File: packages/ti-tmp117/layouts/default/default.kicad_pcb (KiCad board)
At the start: 2 copper layers, 4 parts

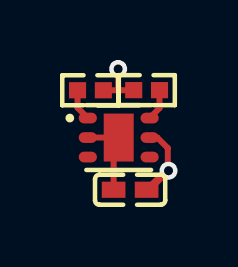
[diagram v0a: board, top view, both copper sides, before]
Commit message: rebuild all packages
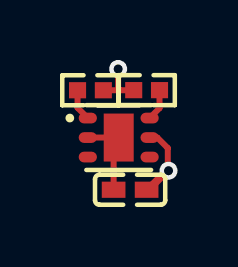
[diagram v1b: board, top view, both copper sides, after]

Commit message: Rename pjrc-teensy_4_1 to pjrc-teensy-4-1
- Renamed package directory from pjrc-teensy_4_1 to pjrc-teensy-4-1
- Updated package naming convention to use hyphens instead of underscores
- Package marked as 'Done' in package-todos.md
- Fixed formatting issues (end-of-file and trailing whitespace)
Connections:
- net gnd renamed GND
- net hv renamed VCC
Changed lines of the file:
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@@
     )
     (net 0 "")
-    (net 1 "gnd")
+    (net 1 "GND")
     (net 2 "ALERT")
     (net 3 "ADD0")
-    (net 4 "hv")
+    (net 4 "VCC")
     (net 5 "SDA")
     (net 6 "SCL")
@@
             (at 0 0 0)
             (layer "User.9")
-            (hide yes)
-            (effects
-                (font
-                    (size 0.125 0.125)
-                    (thickness 0.01875)
-                )
-            )
-        )
-        (property "__atopile_lib_fp_hash__" "8abb505c-885f-7f6b-d492-05175d6245b7"
+            (hide no)
+            (effects
+                (font
+                    (size 0.125 0.125)
+                    (thickness 0.01875)
+                )
+                (hide yes)
+            )
+        )
+        (property "__atopile_lib_fp_hash__" "3d0b050a-bcab-1e74-e762-9705fa715dbf"
             (at 0 0 0)
             (layer "User.9")
@@
             (layer "F.Fab")
         )
+        (fp_text user "%R"
+            (at 0 0 0)
+            (layer "F.Fab")
+            (effects
+                (font
+                    (size 1 1)
+                    (thickness 0.15)
+                )
+            )
+            (unlocked no)
+        )
         (fp_text user "${REFERENCE}"
             (at 0 -4.65 0)
             (layer "F.SilkS")
-            (hide yes)
             (effects
                 (font
@@
             (unlocked no)
         )
-        (fp_text user "${REFERENCE}"
-            (at 0 0 0)
-            (layer "F.Fab")
-            (hide yes)
-            (effects
-                (font
-                    (size 1 1)
-                    (thickness 0.15)
-                )
-                (hide yes)
-            )
-            (unlocked no)
-        )
         (pad "1" smd oval
-            (at -1.03 -0.65 270)
+            (at -1.03 -0.65 -90)
             (size 0.36 0.61)
-            (layers "F.Cu" "F.Mask" "F.Paste")
+            (layers "F.Cu" "F.Paste" "F.Mask")
             (net 6 "SCL")
         )
         (pad "2" smd oval
-            (at -1.03 0 270)
+            (at -1.03 0 -90)
             (size 0.36 0.61)
-            (layers "F.Cu" "F.Mask" "F.Paste")
-            (net 1 "gnd")
+            (layers "F.Cu" "F.Paste" "F.Mask")
+            (net 1 "GND")
         )
         (pad "3" smd oval
-            (at -1.03 0.65 270)
+            (at -1.03 0.65 -90)
             (size 0.36 0.61)
-            (layers "F.Cu" "F.Mask" "F.Paste")
+            (layers "F.Cu" "F.Paste" "F.Mask")
             (net 2 "ALERT")
         )
         (pad "4" smd oval
-            (at 1.03 0.65 270)
+            (at 1.03 0.65 -90)
             (size 0.36 0.61)
-            (layers "F.Cu" "F.Mask" "F.Paste")
+            (layers "F.Cu" "F.Paste" "F.Mask")
             (net 3 "ADD0")
         )
         (pad "5" smd oval
-            (at 1.03 0 270)
+            (at 1.03 0 -90)
             (size 0.36 0.61)
-            (layers "F.Cu" "F.Mask" "F.Paste")
-            (net 4 "hv")
+            (layers "F.Cu" "F.Paste" "F.Mask")
+            (net 4 "VCC")
         )
         (pad "6" smd oval
-            (at 1.03 -0.65 270)
+            (at 1.03 -0.65 -90)
             (size 0.36 0.61)
-            (layers "F.Cu" "F.Mask" "F.Paste")
+            (layers "F.Cu" "F.Paste" "F.Mask")
             (net 5 "SDA")
         )
@@
             (at 0 0 0)
             (size 1 1.6)
-            (layers "F.Cu" "F.Mask" "F.Paste")
-            (net 1 "gnd")
-        )
-        (embedded_fonts no)
+            (layers "F.Cu" "F.Paste" "F.Mask")
+            (net 1 "GND")
+        )
         (model "${KIPRJMOD}/../../parts/Texas_Instruments_TMP117AIDRVR/WSON-6_L2.0-W2.0-H0.8-P0.65.step"
             (offset
@@
             )
         )
-        (property "__atopile_lib_fp_hash__" "cd0f5f87-a8ae-b8be-c38c-27e3a9632768"
+        (property "__atopile_lib_fp_hash__" "ac993d00-cd2e-9909-323a-aafc825a9032"
             (at 0 0 0)
             (layer "User.9")
@@
             (size 0.57 0.54)
             (layers "F.Cu" "F.Paste" "F.Mask")
-            (net 4 "hv")
+            (net 4 "VCC")
         )
         (pad "1" smd rect
@@
             )
         )
-        (property "__atopile_lib_fp_hash__" "cd0f5f87-a8ae-b8be-c38c-27e3a9632768"
+        (property "__atopile_lib_fp_hash__" "ac993d00-cd2e-9909-323a-aafc825a9032"
             (at 0 0 0)
             (layer "User.9")
@@
             (size 0.57 0.54)
             (layers "F.Cu" "F.Paste" "F.Mask")
-            (net 4 "hv")
+            (net 4 "VCC")
         )
         (pad "1" smd rect
@@
             )
         )
-        (property "__atopile_lib_fp_hash__" "06cb3746-9f81-d057-81ed-4514f27d7e2a"
+        (property "__atopile_lib_fp_hash__" "f8a97365-7255-729e-24e5-6102db053d76"
             (at 0 0 0)
             (layer "User.9")
@@
             (size 0.79 0.54)
             (layers "F.Cu" "F.Paste" "F.Mask")
-            (net 1 "gnd")
+            (net 1 "GND")
         )
         (pad "1" smd rect
@@
             (size 0.79 0.54)
             (layers "F.Cu" "F.Paste" "F.Mask")
-            (net 4 "hv")
+            (net 4 "VCC")
         )
         (model "${KIPRJMOD}/../../parts/Samsung_Electro_Mechanics_CL05B104KO5NNNC/C0402_L1.0-W0.5-H0.5.step"
